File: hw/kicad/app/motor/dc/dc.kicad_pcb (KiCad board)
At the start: 2 copper layers, 50 x 50 mm, 22 parts, among them J1 TOP, J2 Motor 1, J3 Motor 2, J4 Motor 3, J5 Motor 4, J6 BOTTUM, U1 DRV8870DDA, U2 DRV8870DDA, U3 DRV8870DDA, U4 DRV8870DDA

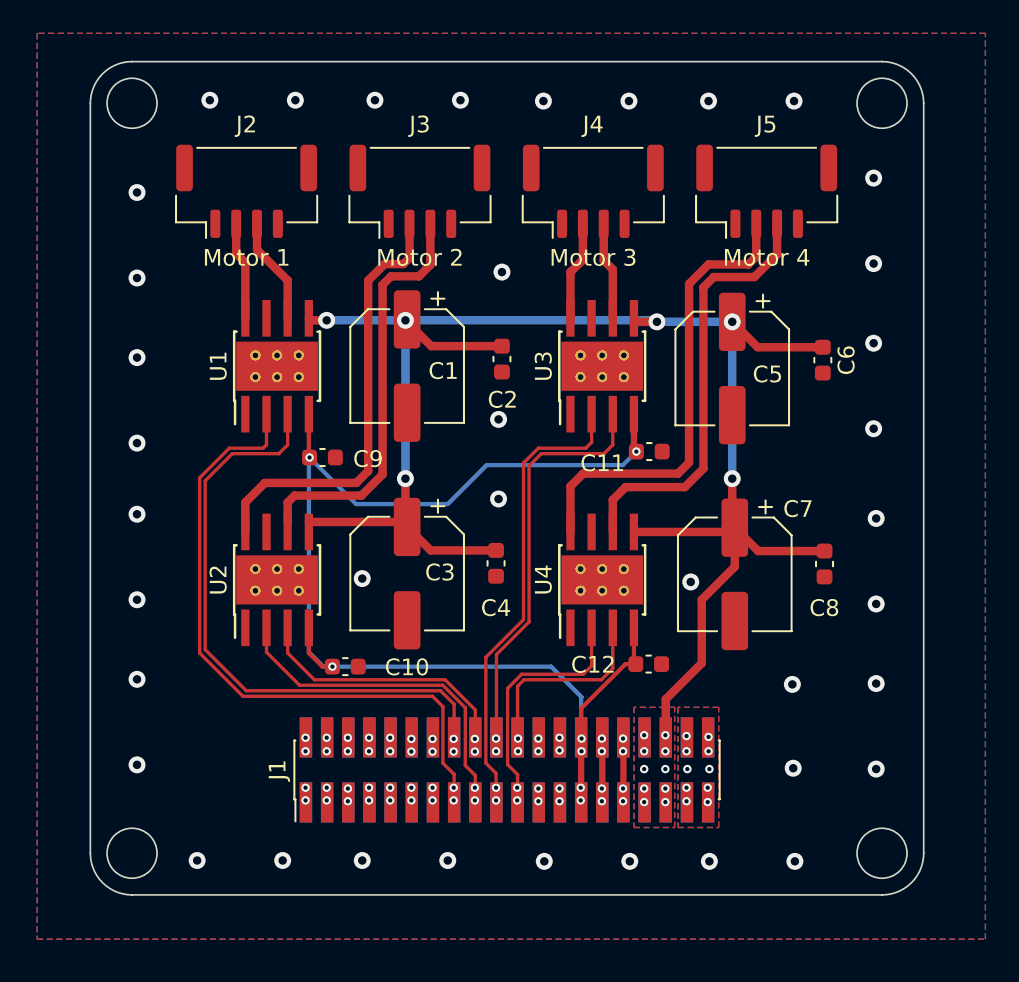
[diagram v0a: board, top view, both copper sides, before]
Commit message: 修改尺寸至45x45
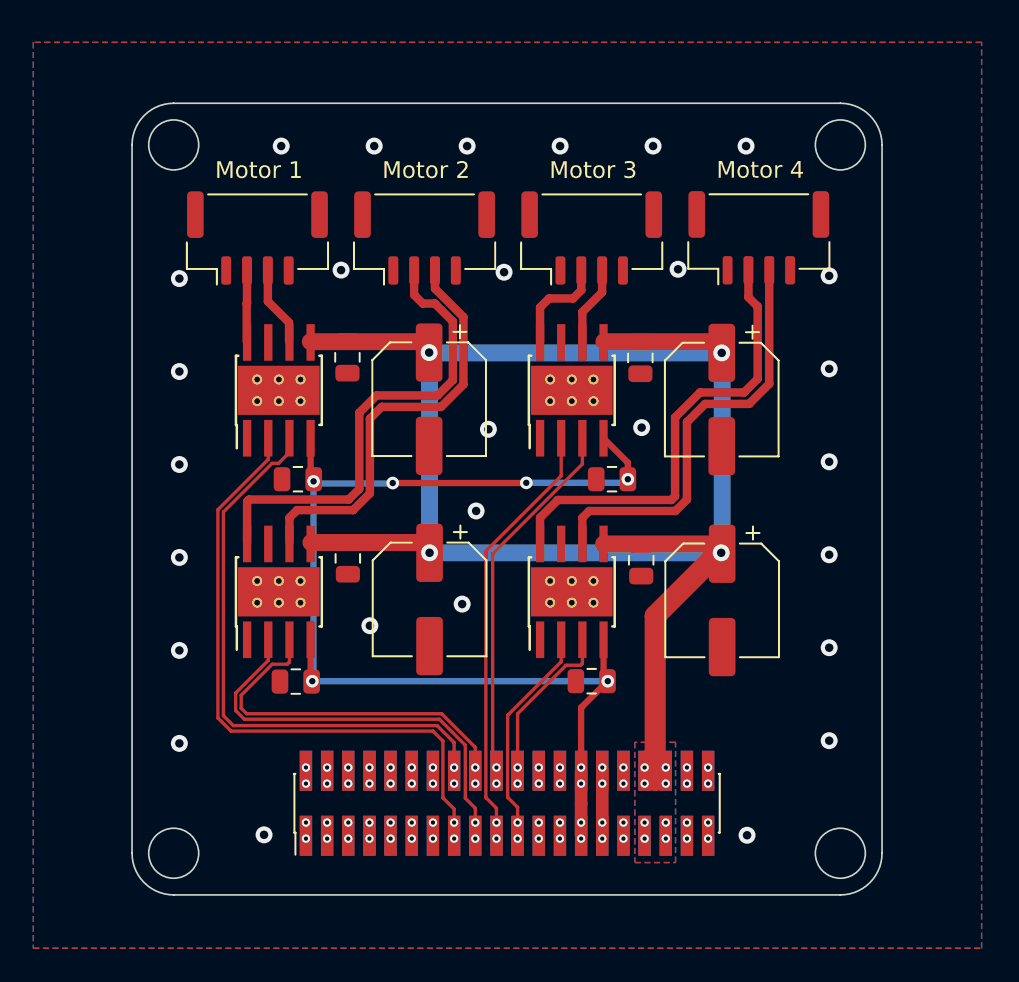
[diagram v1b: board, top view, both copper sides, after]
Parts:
- C10, C11, C12, C2, C4, C6, C8, C9: footprint Capacitor_SMD:C_0603_1608Metric -> Capacitor_SMD:C_0805_2012Metric
- moved C8 11.0 mm to (83.8, 60.6)
- moved C6 10.9 mm to (83.7, 48.5)
- moved C2 9.27 mm to (66.1, 48.5)
- moved C4 8.89 mm to (66.2, 60.5)
- moved C12 3.57 mm to (80.8, 67.9), turned to 180 degrees
- moved C10 3.10 mm to (63.0, 67.9), turned to 180 degrees
- moved J2 2.87 mm to (60.7, 41.3)
- moved J5 2.83 mm to (90.8, 41.3)
- moved J3 2.81 mm to (70.8, 41.3)
- moved J4 2.80 mm to (80.8, 41.3)
- moved C11 2.78 mm to (82.0, 55.8), turned to 180 degrees
- moved C1 2.39 mm to (71.0, 51.0)
- moved U3 2.33 mm to (79.6, 50.4)
- moved C3 2.05 mm to (71.1, 63.0)
- moved J1 2.00 mm to (75.7, 75.2)
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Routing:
- net /PWM_4: track 16.4 -> 22.3 mm
- net /PWM_3: track 21.3 -> 25.5 mm
- net GND: track 3.84 -> 0.00 mm, vias 53 -> 40
- net +3.3V: track 74.6 -> 71.4 mm, vias 7 -> 10
- net /PWM_6: track 24.5 -> 22.3 mm
- net /OUT3: track 26.4 -> 28.4 mm
- net /PWM_5: track 27.7 -> 26.0 mm
- net /PWM_8: track 11.7 -> 9.98 mm
- net /OUT2: track 6.44 -> 4.79 mm
- net /PWM_7: track 15.0 -> 13.3 mm
- net /OUT1: track 5.90 -> 4.27 mm
- net /PWM_2: track 36.1 -> 34.7 mm
- net /OUT6: track 5.89 -> 4.81 mm
- net /PWM_1: track 39.1 -> 38.1 mm
- net /OUT4: track 24.8 -> 25.4 mm
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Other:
- board size 50 x 50 mm -> 45 x 47.5 mm
